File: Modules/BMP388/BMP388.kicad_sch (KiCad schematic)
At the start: 3 parts, among them U1 BMP388

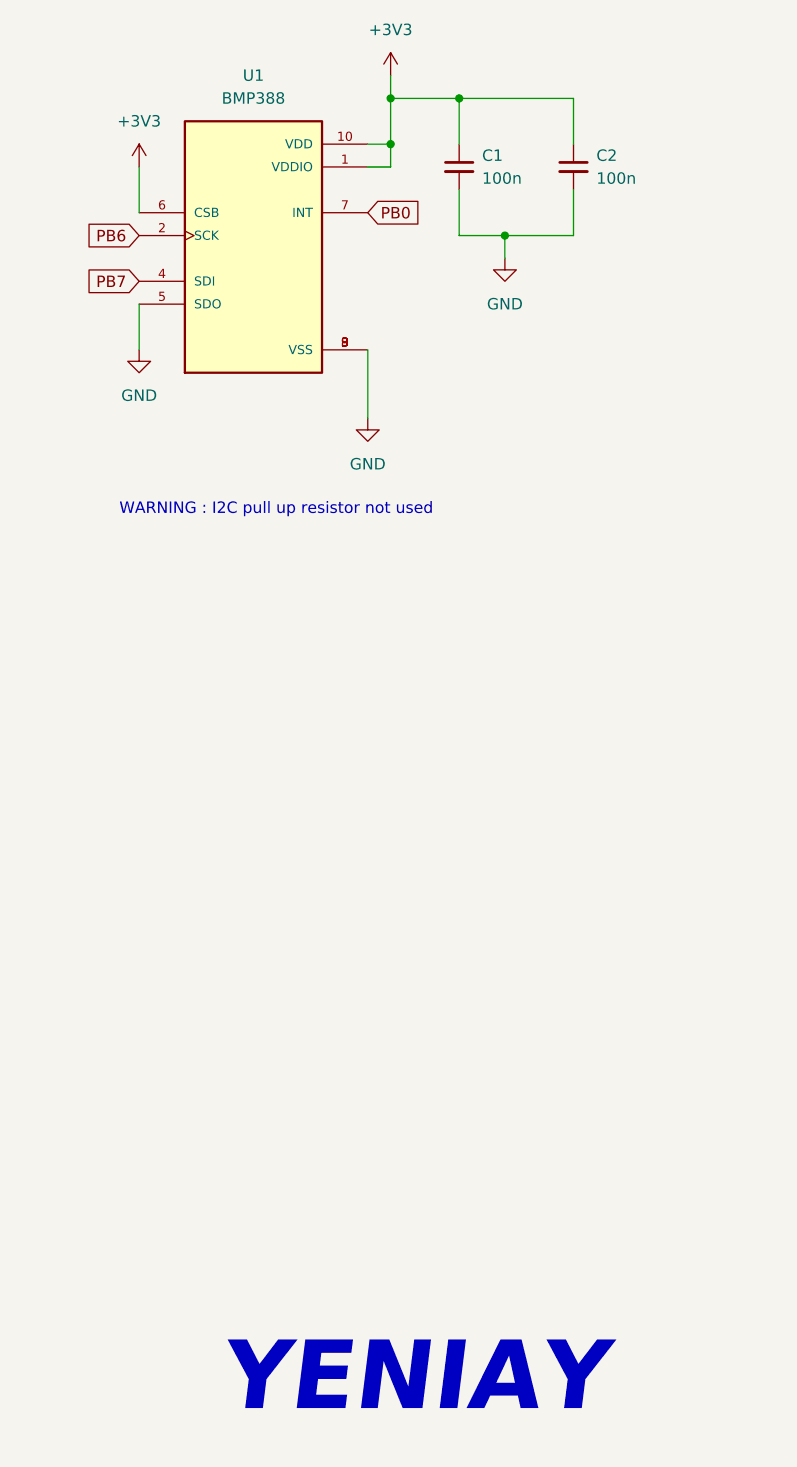
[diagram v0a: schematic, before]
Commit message: BMP388 updated.
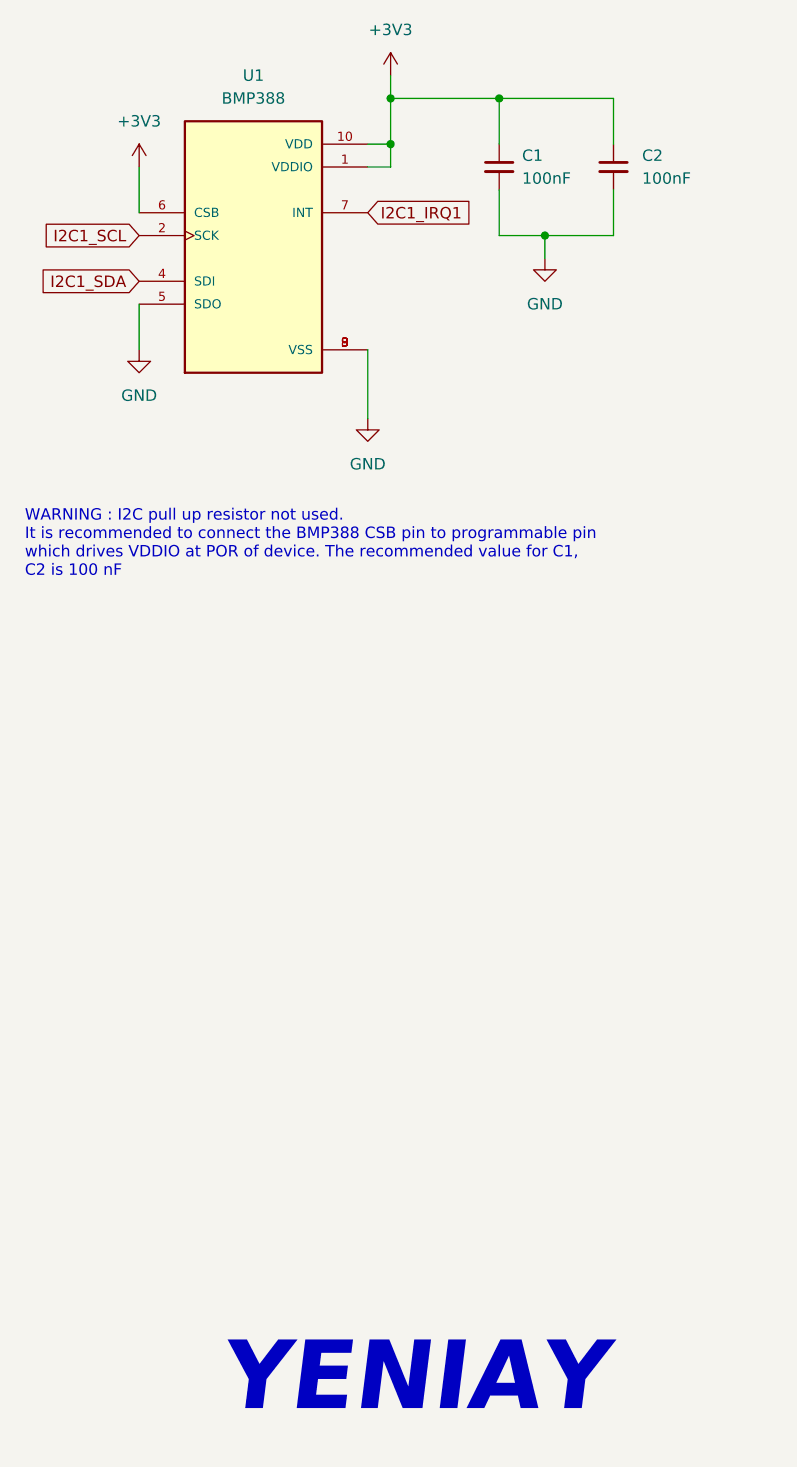
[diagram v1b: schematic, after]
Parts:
- C1, C2: value 100n -> 100nF
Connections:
- net PB0 renamed I2C1_IRQ1 
- net PB6 renamed I2C1_SCL 
- net PB7 renamed I2C1_SDA 
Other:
- note added: "WARNING : I2C pull up resistor not used. It is recommended to connect the BMP388 CSB pin to programmable pin which drives VDDIO at POR of device. The recommended value for C1, C2 is 100 nF"
- note removed: "WARNING : I2C pull up resistor not used"
- moved on the sheet: C1, C2
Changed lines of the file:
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@@
 	)
 	(junction
-		(at 116.84 119.38)
+		(at 121.285 119.38)
 		(diameter 0)
 		(color 0 0 0 0)
@@
 	)
 	(junction
-		(at 121.92 134.62)
+		(at 126.365 134.62)
 		(diameter 0)
 		(color 0 0 0 0)
@@
 	(wire
 		(pts
-			(xy 116.84 129.54) (xy 116.84 134.62)
-		)
-		(stroke
-			(width 0)
-			(type default)
-		)
-	)
-	(wire
-		(pts
-			(xy 121.92 134.62) (xy 121.92 137.16)
-		)
-		(stroke
-			(width 0)
-			(type default)
-		)
-	)
-	(wire
-		(pts
-			(xy 129.54 129.54) (xy 129.54 134.62)
-		)
-		(stroke
-			(width 0)
-			(type default)
-		)
-	)
-	(wire
-		(pts
-			(xy 116.84 124.46) (xy 116.84 119.38)
+			(xy 121.285 129.54) (xy 121.285 134.62)
+		)
+		(stroke
+			(width 0)
+			(type default)
+		)
+	)
+	(wire
+		(pts
+			(xy 126.365 134.62) (xy 126.365 137.16)
+		)
+		(stroke
+			(width 0)
+			(type default)
+		)
+	)
+	(wire
+		(pts
+			(xy 133.985 129.54) (xy 133.985 134.62)
+		)
+		(stroke
+			(width 0)
+			(type default)
+		)
+	)
+	(wire
+		(pts
+			(xy 121.285 124.46) (xy 121.285 119.38)
+		)
+		(stroke
+			(width 0)
+			(type default)
+		)
+	)
+	(wire
+		(pts
+			(xy 109.22 119.38) (xy 121.285 119.38)
 		)
 		(stroke
@@
 	(wire
 		(pts
-			(xy 121.92 134.62) (xy 129.54 134.62)
+			(xy 126.365 134.62) (xy 133.985 134.62)
 		)
 		(stroke
@@
 	(wire
 		(pts
-			(xy 116.84 134.62) (xy 121.92 134.62)
+			(xy 121.285 134.62) (xy 126.365 134.62)
 		)
 		(stroke
@@
 	(wire
 		(pts
-			(xy 129.54 124.46) (xy 129.54 119.38)
+			(xy 133.985 124.46) (xy 133.985 119.38)
 		)
 		(stroke
@@
 	(wire
 		(pts
-			(xy 109.22 119.38) (xy 116.84 119.38)
-		)
-		(stroke
-			(width 0)
-			(type default)
-		)
-	)
-	(wire
-		(pts
-			(xy 116.84 119.38) (xy 129.54 119.38)
+			(xy 121.285 119.38) (xy 133.985 119.38)
 		)
 		(stroke
@@
 		)
 	)
-	(text "WARNING : I2C pull up resistor not used"
+	(text "WARNING : I2C pull up resistor not used.\nIt is recommended to connect the BMP388 CSB pin to programmable pin\nwhich drives VDDIO at POR of device. The recommended value for C1, \nC2 is 100 nF"
 		(exclude_from_sim no)
-		(at 96.52 165.1 0)
+		(at 68.58 168.91 0)
 		(effects
 			(font
 				(size 1.27 1.27)
 			)
-		)
-	)
-	(global_label "PB0"
+			(justify left)
+		)
+	)
+	(global_label "I2C1_IRQ1 "
 		(shape input)
 		(at 106.68 132.08 0)
@@
 		)
 		(property "Intersheetrefs" "${INTERSHEET_REFS}"
-			(at 113.4147 132.08 0)
+			(at 120.309 132.08 0)
 			(effects
 				(font
@@
 		)
 	)
-	(global_label "PB6"
+	(global_label "I2C1_SCL "
 		(shape input)
 		(at 81.28 134.62 180)
@@
 		)
 		(property "Intersheetrefs" "${INTERSHEET_REFS}"
-			(at 74.5453 134.62 0)
+			(at 68.5582 134.62 0)
 			(effects
 				(font
@@
 		)
 	)
-	(global_label "PB7"
+	(global_label "I2C1_SDA "
 		(shape input)
 		(at 81.28 139.7 180)
@@
 		)
 		(property "Intersheetrefs" "${INTERSHEET_REFS}"
-			(at 74.5453 139.7 0)
+			(at 68.4977 139.7 0)
 			(effects
 				(font
@@
 	(symbol
 		(lib_id "Device:C_Small")
-		(at 129.54 127 0)
+		(at 133.985 127 0)
 		(unit 1)
 		(exclude_from_sim no)
@@
 		(fields_autoplaced yes)
 		(property "Reference" "C2"
-			(at 132.08 125.7362 0)
+			(at 137.16 125.7362 0)
 			(effects
 				(font
@@
 			)
 		)
-		(property "Value" "100n"
-			(at 132.08 128.2762 0)
+		(property "Value" "100nF"
+			(at 137.16 128.2762 0)
 			(effects
 				(font
@@
 		)
 		(property "Footprint" ""
-			(at 129.54 127 0)
+			(at 133.985 127 0)
 			(effects
 				(font
@@
 		)
 		(property "Datasheet" "~"
-			(at 129.54 127 0)
+			(at 133.985 127 0)
 			(effects
 				(font
@@
 		)
 		(property "Description" "Unpolarized capacitor, small symbol"
-			(at 129.54 127 0)
+			(at 133.985 127 0)
 			(effects
 				(font
@@
 	(symbol
 		(lib_id "Device:C_Small")
-		(at 116.84 127 0)
+		(at 121.285 127 0)
 		(unit 1)
 		(exclude_from_sim no)
@@
 		(dnp no)
 		(property "Reference" "C1"
-			(at 119.38 125.7362 0)
+			(at 123.825 125.7362 0)
 			(effects
 				(font
@@
 			)
 		)
-		(property "Value" "100n"
-			(at 119.38 128.2762 0)
+		(property "Value" "100nF"
+			(at 123.825 128.2762 0)
 			(effects
 				(font
@@
 		)
 		(property "Footprint" ""
-			(at 116.84 127 0)
+			(at 121.285 127 0)
 			(effects
 				(font
@@
 		)
 		(property "Datasheet" "~"
-			(at 116.84 127 0)
+			(at 121.285 127 0)
 			(effects
 				(font
@@
 		)
 		(property "Description" "Unpolarized capacitor, small symbol"
-			(at 116.84 127 0)
+			(at 121.285 127 0)
 			(effects
 				(font
@@
 	(symbol
 		(lib_id "power:GND")
-		(at 121.92 137.16 0)
+		(at 126.365 137.16 0)
 		(unit 1)
 		(exclude_from_sim no)
@@
 		(fields_autoplaced yes)
 		(property "Reference" "#PWR05"
-			(at 121.92 143.51 0)
+			(at 126.365 143.51 0)
 			(effects
 				(font
@@
 		)
 		(property "Value" "GND"
-			(at 121.92 142.24 0)
+			(at 126.365 142.24 0)
 			(effects
 				(font
@@
 		)
 		(property "Footprint" ""
-			(at 121.92 137.16 0)
+			(at 126.365 137.16 0)
 			(effects
 				(font
@@
 		)
 		(property "Datasheet" ""
-			(at 121.92 137.16 0)
+			(at 126.365 137.16 0)
 			(effects
 				(font
@@
 		)
 		(property "Description" "Power symbol creates a global label with name \"GND\" , ground"
-			(at 121.92 137.16 0)
-			(effects
-				(font
+			(at 126.365 137.16 0)
+			(effects
+				(font
